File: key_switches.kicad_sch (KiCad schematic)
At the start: 28 parts, among them SW1 SW_Push, SW10 SW_Push, SW11 SW_Push, SW12 SW_Push, SW13 SW_Push, SW14 SW_Push, SW2 SW_Push, SW3 SW_Push, SW4 SW_Push, SW5 SW_Push, SW6 SW_Push, SW7 SW_Push, SW8 SW_Push, SW9 SW_Push

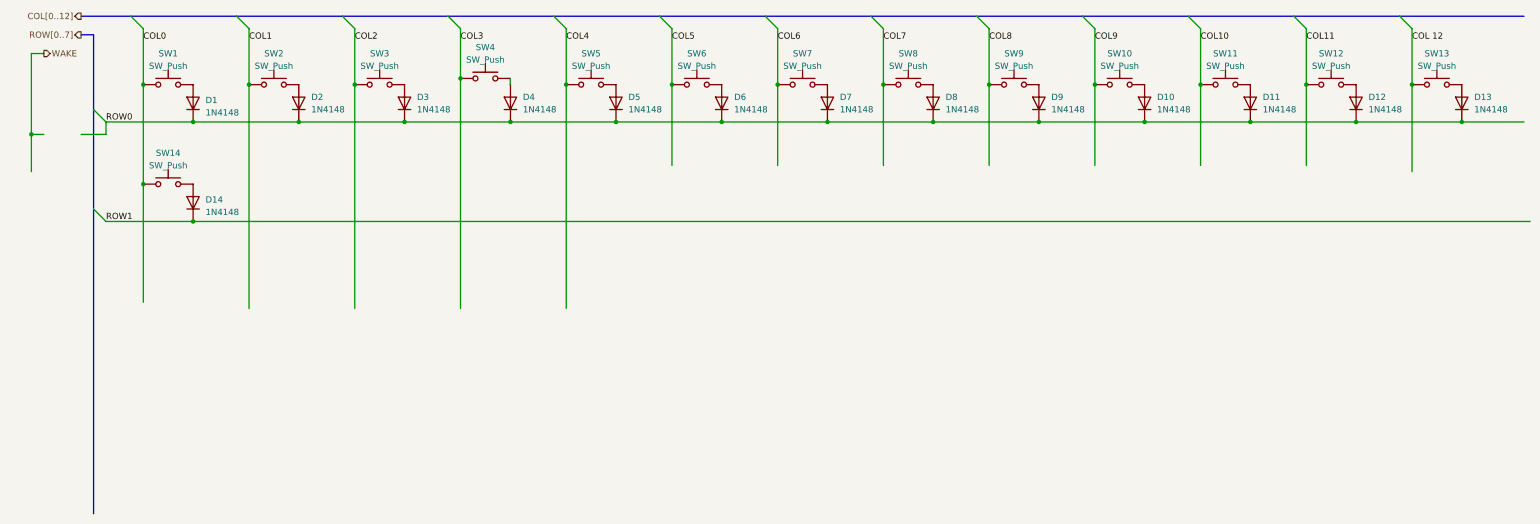
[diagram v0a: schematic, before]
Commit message: more changes to keys
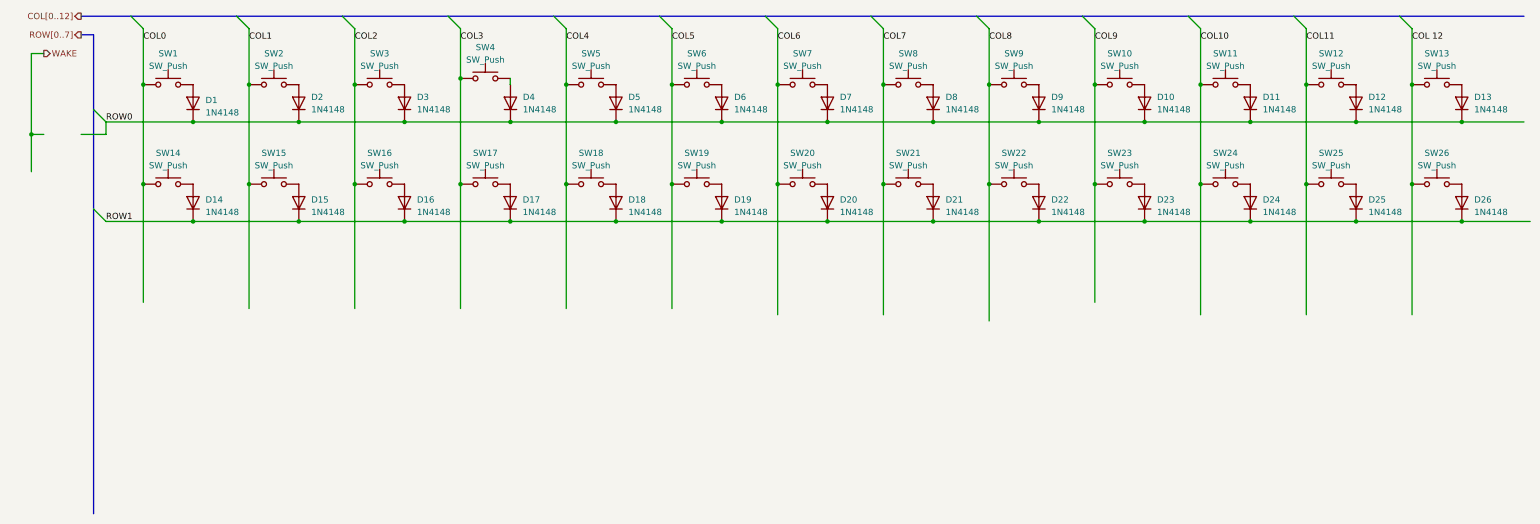
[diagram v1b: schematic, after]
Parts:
- added D15, D16, D17, D18, D19, D20, D21, D22, D23, D24, D25, D26: 1N4148, Diode_THT:D_DO-35_SOD27_P7.62mm_Horizontal, symbol Diode:1N4148
- added SW15, SW16, SW17, SW18, SW19, SW20, SW21, SW22, SW23, SW24, SW25, SW26: SW_Push, symbol Switch:SW_Push
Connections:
- net COL 12: now also SW26.1
- net COL1: now also SW15.1
- net COL10: now also SW24.1
- net COL11: now also SW25.1
- net COL2: now also SW16.1
- net COL3: now also SW17.1
- net COL4: now also SW18.1
- net COL5: now also SW19.1
- net COL6: now also SW20.1
- net COL7: now also SW21.1
- net COL8: now also SW22.1
- net COL9: now also SW23.1
- net ROW1: now also D15.1 (K), D16.1 (K), D17.1 (K), D18.1 (K), D19.1 (K), D20.1 (K), D21.1 (K), D22.1 (K), D23.1 (K), D24.1 (K), D25.1 (K), D26.1 (K)
- new net: D20.2 (A), SW20.2
- new net: D17.2 (A), SW17.2
- new net: D15.2 (A), SW15.2
- new net: D23.2 (A), SW23.2
- new net: D21.2 (A), SW21.2
- new net: D19.2 (A), SW19.2
- new net: D18.2 (A), SW18.2
- new net: D24.2 (A), SW24.2
- new net: D22.2 (A), SW22.2
- new net: D25.2 (A), SW25.2
- new net: D16.2 (A), SW16.2
- new net: D26.2 (A), SW26.2
